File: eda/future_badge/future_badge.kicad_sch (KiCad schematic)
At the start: 9 parts

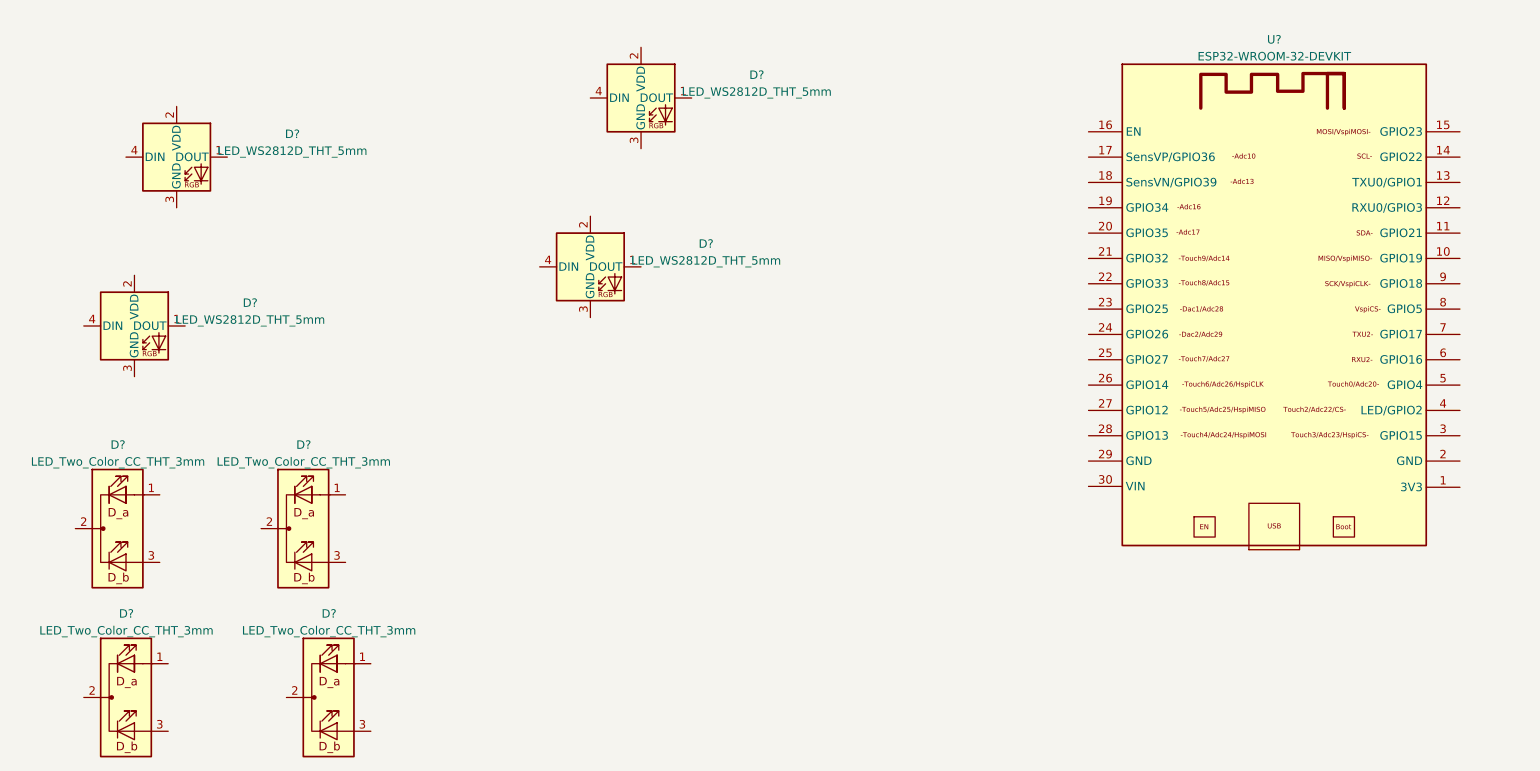
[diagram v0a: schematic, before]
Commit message: updated schematic
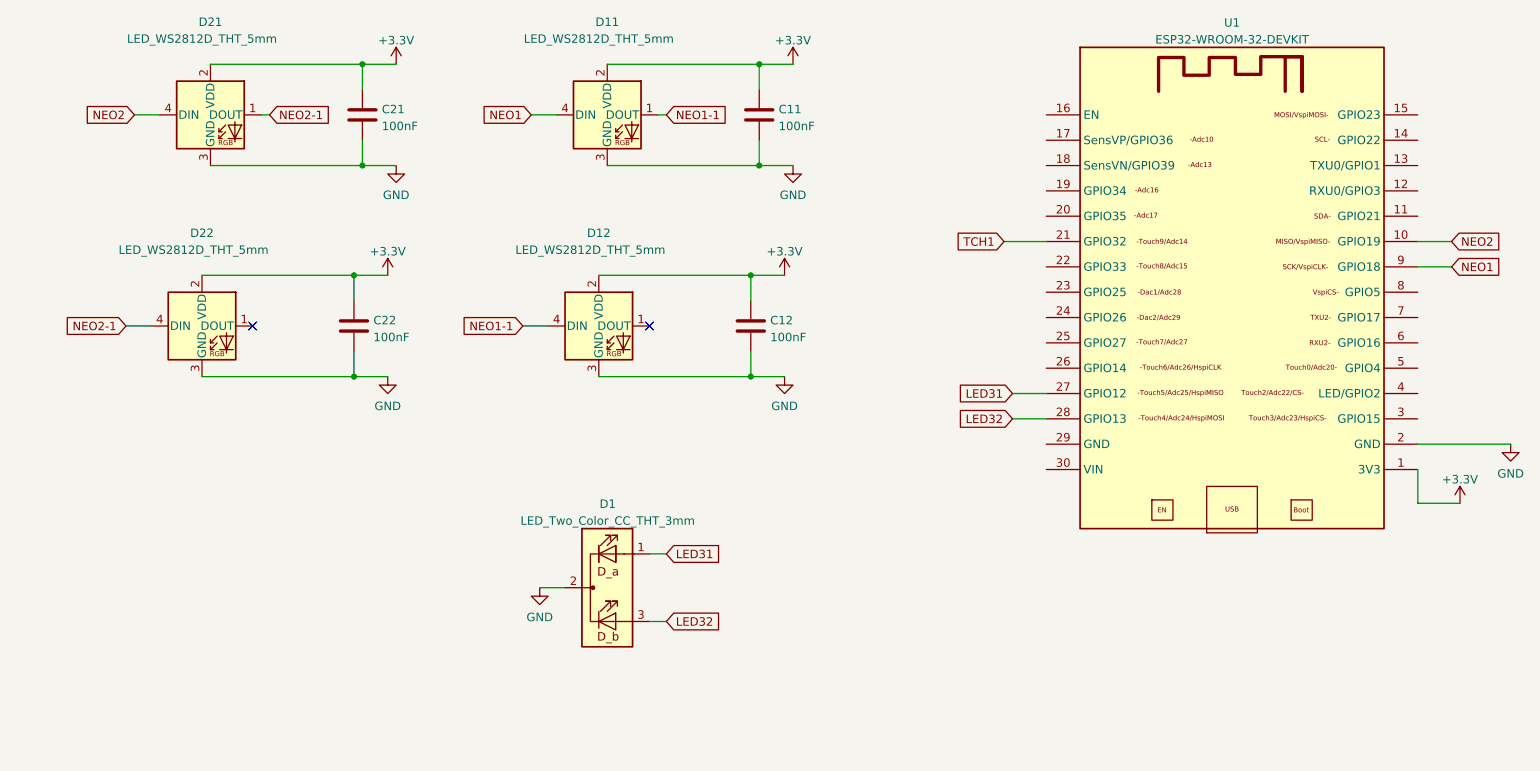
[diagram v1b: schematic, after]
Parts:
- removed D? (x3): LED_Two_Color_CC_THT_3mm, 0_local:LED_D3.0mm-3-TwoColor_backsilk, symbol 0_local:LED_Two_Color_CC_THT_3mm
- removed D? (x3): LED_WS2812D_THT_5mm, 0_local:LED_D5.0mm-4_WS2812D_front, symbol 0_local:LED_WS2812D_THT_5mm
- removed U?: ESP32-WROOM-32-DEVKIT, 0_local:ESP32_DEVKIT_V1, symbol 0_local:ESP32-WROOM-32-DEVKIT
- added C11, C12, C21, C22: 100nF, 0_local:C_Disc_D3.0mm_W2.0mm_P2.50mm_backsilk, symbol 0_local:C_Disc_D3
- added D12, D21, D22: LED_WS2812D_THT_5mm, 0_local:LED_D5.0mm-4_WS2812D_front, symbol 0_local:LED_WS2812D_THT_5mm
- added U1: ESP32-WROOM-32-DEVKIT, 0_local:ESP32_DEVKIT_V1, symbol 0_local:ESP32-WROOM-32-DEVKIT
- gave numbers to parts that had none: 2
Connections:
- net LED31: now reaches D1.1 (RA)
- net LED31: now also U1.27 (GPIO12)
- net GND: now reaches D1.2 (K)
- net GND: now also D11.3 (GND), C11.2, C12.2, C21.2, C22.2, D12.3 (GND), D21.3 (GND), D22.3 (GND), U1.2 (GND)
- net LED32: now reaches D1.3 (BA)
- net LED32: now also U1.28 (GPIO13)
- net NEO1-1: now reaches D11.1 (DOUT)
- net NEO1-1: now also D12.4 (DIN)
- net +3.3V: now reaches D11.2 (VDD)
- net +3.3V: now also C11.1, C12.1, C21.1, C22.1, D12.2 (VDD), D21.2 (VDD), D22.2 (VDD), U1.1 (3V3)
- net NEO1: now reaches D11.4 (DIN)
- net NEO1: now also U1.9 (GPIO18)
- new net NEO2: D21.4 (DIN), U1.10 (GPIO19)
- new net NEO2-1: D21.1 (DOUT), D22.4 (DIN)
- new net TCH1: U1.21 (GPIO32)
- no-connect marks 0 -> 2
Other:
- moved on the sheet: D1, D11
